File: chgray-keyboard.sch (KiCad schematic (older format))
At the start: 1 part

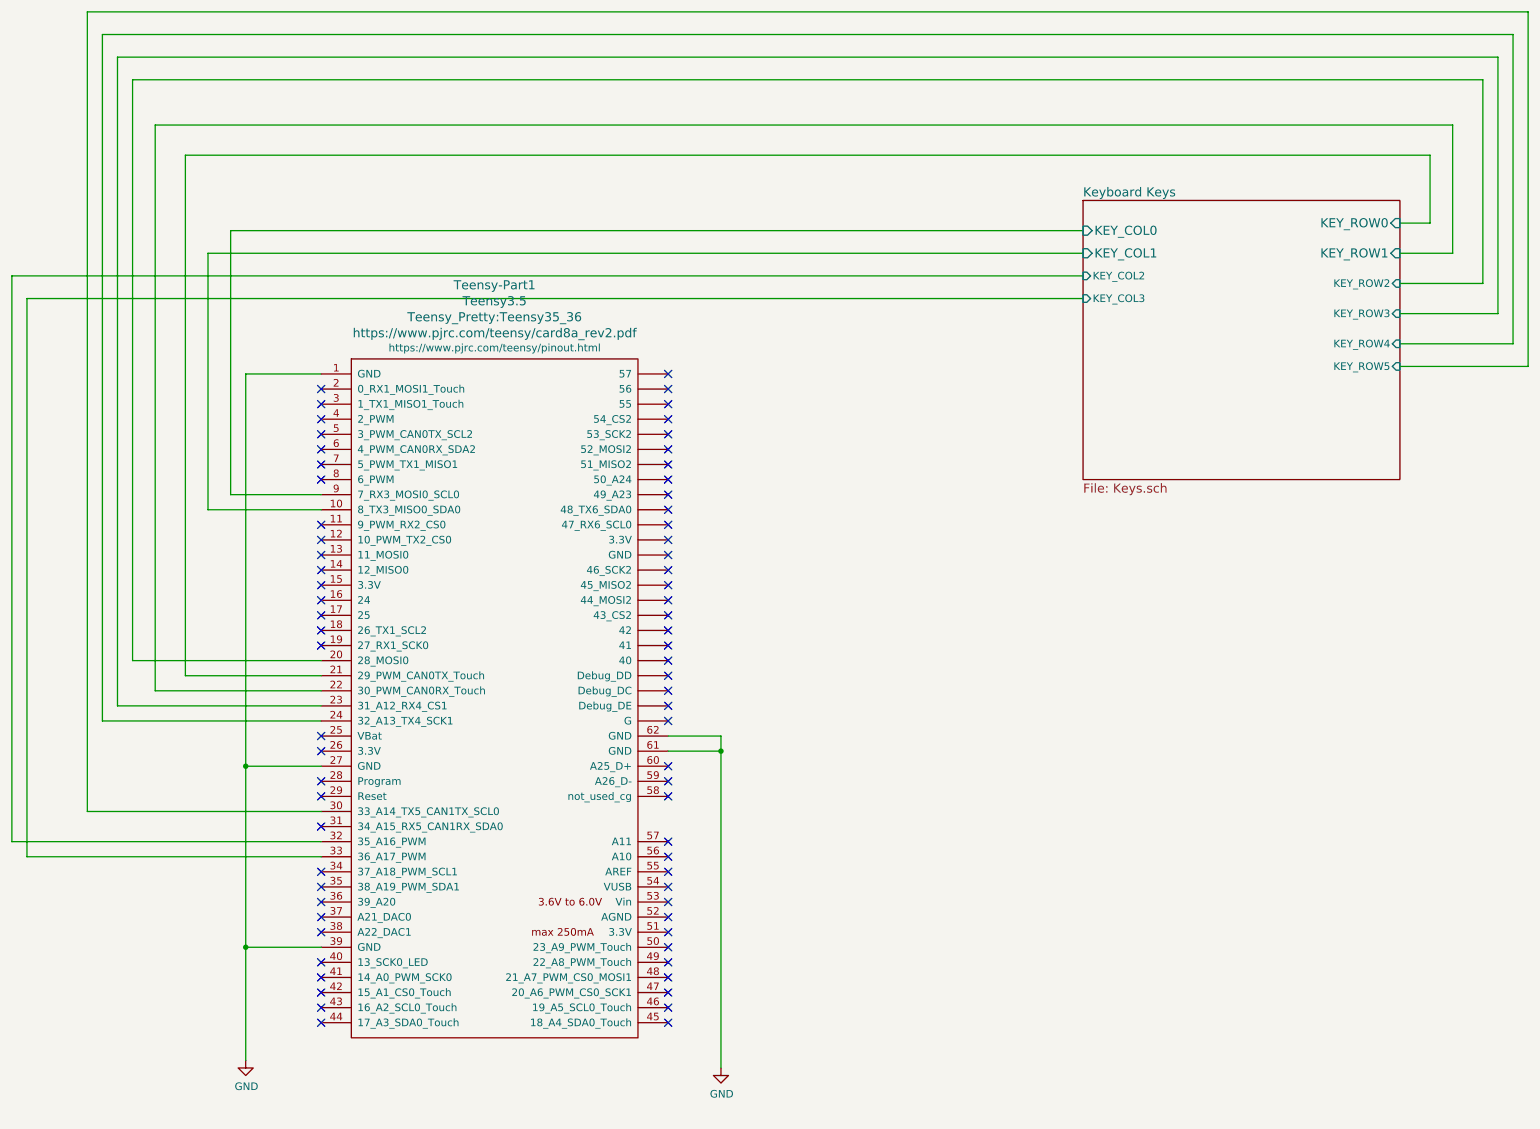
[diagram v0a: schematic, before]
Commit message: might work...
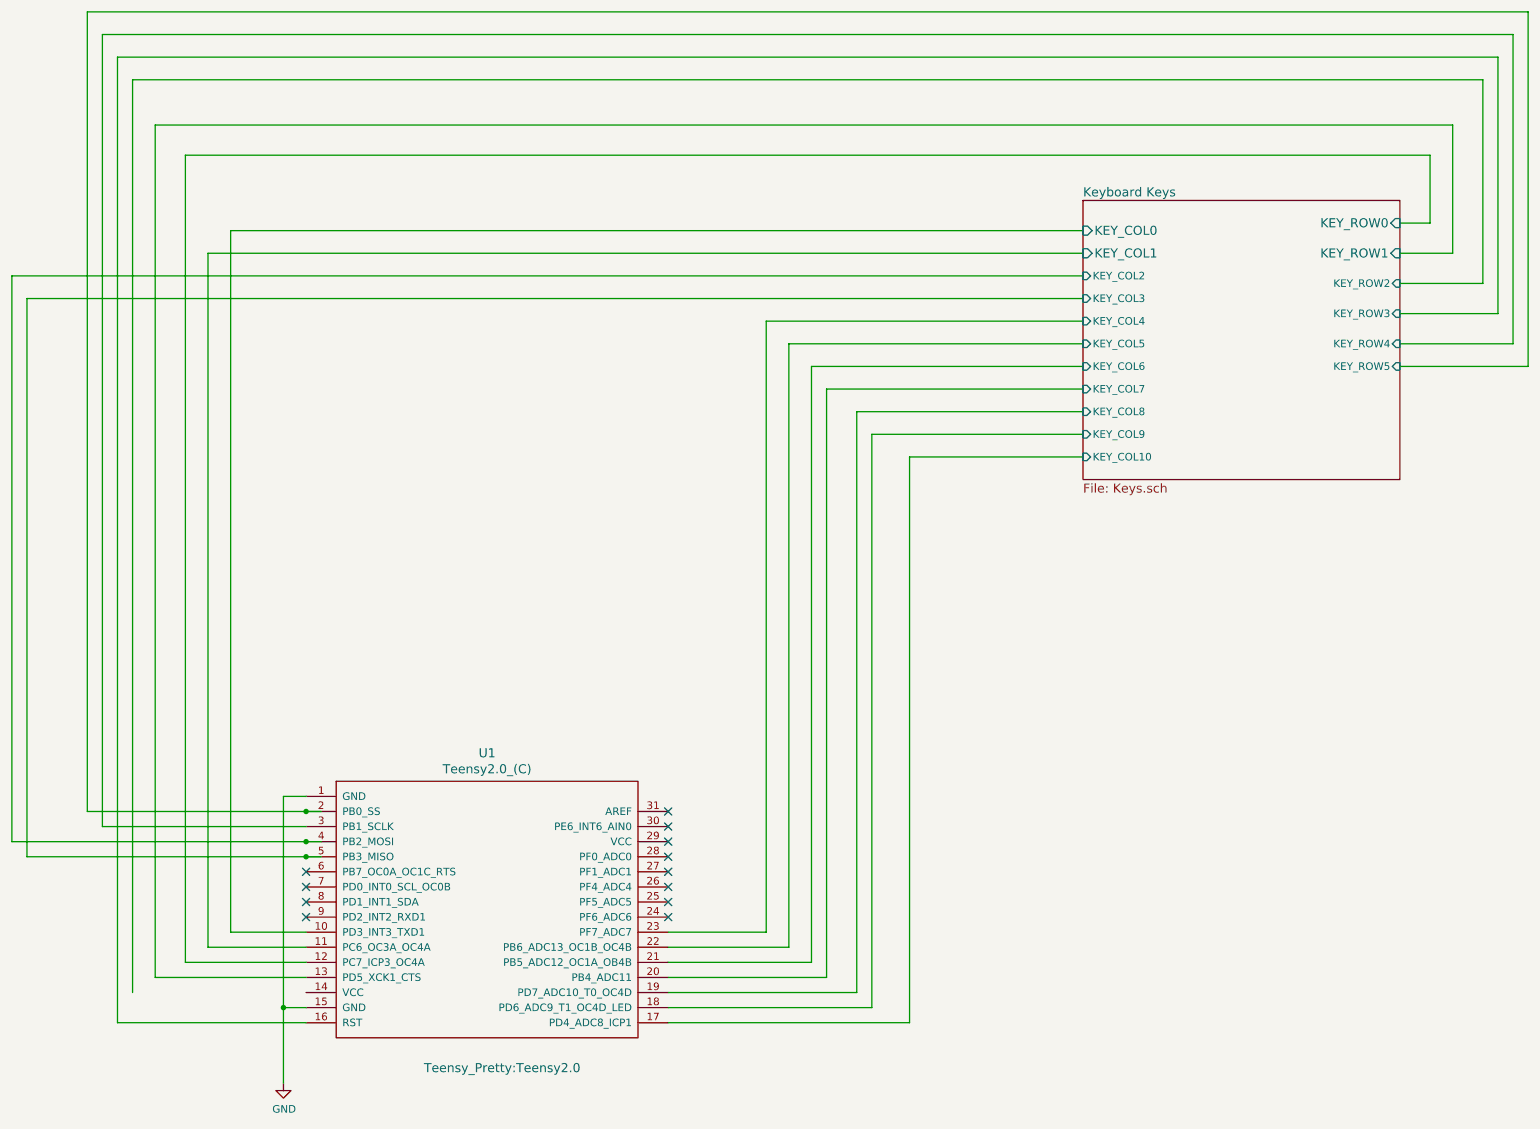
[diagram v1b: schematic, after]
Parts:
- removed Teensy-Part1: Teensy3.5, Teensy_Pretty:Teensy35_36, symbol chgray-keyboard-rescue:Teensy3.5-Teensy
- added U1: Teensy2.0_(C), Teensy_Pretty:Teensy2.0, symbol Teensy:Teensy2.0_(C)
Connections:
- wire segments 52 -> 69
- no-connect marks 71 -> 12
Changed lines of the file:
@@
 F10 "KEY_COL2" I L 7300 2300 50
 F11 "KEY_COL3" I L 7300 2450 50
+F12 "KEY_COL4" I L 7300 2600 50
+F13 "KEY_COL5" I L 7300 2750 50
+F14 "KEY_COL6" I L 7300 2900 50
+F15 "KEY_COL7" I L 7300 3050 50
+F16 "KEY_COL8" I L 7300 3200 50
+F17 "KEY_COL9" I L 7300 3350 50
+F18 "KEY_COL10" I L 7300 3500 50
 $EndSheet
 Wire Wire Line
@@
 	9600 1500 1350 1500
 Wire Wire Line
-	1350 1500 1350 4950
-Wire Wire Line
-	1150 5050 1150 1300
-Wire Wire Line
 	1150 1300 9750 1300
 Wire Wire Line
 	9750 1300 9750 2150
-Wire Wire Line
-	1350 4950 2250 4950
-Wire Wire Line
-	2250 5050 1150 5050
 Wire Wire Line
 	7300 2000 1650 2000
@@
 Wire Wire Line
 	9400 1950 9600 1950
-Wire Wire Line
-	1650 2000 1650 3750
-Wire Wire Line
-	1650 3750 2250 3750
-Wire Wire Line
-	2250 3850 1500 3850
-Wire Wire Line
-	1500 3850 1500 2150
 Wire Wire Line
 	1500 2150 7300 2150
@@
 	9950 1000 1000 1000
 Wire Wire Line
-	1000 1000 1000 4850
-Wire Wire Line
-	1000 4850 2250 4850
-NoConn ~ 4550 3850
-NoConn ~ 4550 3950
-NoConn ~ 4550 4050
-NoConn ~ 4550 4250
-NoConn ~ 4550 4350
-NoConn ~ 4550 4450
-NoConn ~ 4550 4550
-NoConn ~ 4550 4750
-NoConn ~ 4550 4850
-NoConn ~ 4550 4950
-NoConn ~ 4550 5050
-NoConn ~ 4550 5150
-NoConn ~ 4550 5250
-NoConn ~ 4550 5550
-NoConn ~ 4550 6050
-NoConn ~ 4550 6150
-NoConn ~ 4550 6250
-NoConn ~ 4550 6350
-NoConn ~ 4550 6450
-NoConn ~ 4550 6550
-NoConn ~ 4550 6650
-NoConn ~ 4550 6750
-NoConn ~ 4550 6850
-NoConn ~ 4550 6950
-NoConn ~ 4550 7050
-NoConn ~ 4550 7150
-NoConn ~ 4550 7250
-NoConn ~ 2250 7250
-NoConn ~ 2250 7150
-NoConn ~ 2250 7050
-NoConn ~ 2250 6950
-NoConn ~ 2250 6850
-NoConn ~ 2250 6650
-NoConn ~ 2250 6550
-NoConn ~ 2250 6450
-NoConn ~ 2250 6350
-NoConn ~ 2250 6250
-NoConn ~ 2250 5950
-NoConn ~ 2250 5750
-NoConn ~ 2250 5650
-NoConn ~ 2250 5450
-NoConn ~ 2250 4550
-NoConn ~ 2250 4650
-NoConn ~ 2250 4750
-NoConn ~ 2250 4450
-NoConn ~ 2250 4350
-NoConn ~ 2250 4250
-NoConn ~ 2250 4150
-NoConn ~ 2250 4050
-NoConn ~ 2250 3950
-NoConn ~ 2250 3650
-NoConn ~ 2250 3050
-NoConn ~ 2250 3150
-NoConn ~ 2250 3250
-NoConn ~ 2250 3350
-NoConn ~ 2250 3450
-NoConn ~ 2250 3550
-Wire Wire Line
 	9400 2550 10050 2550
 Wire Wire Line
@@
 Wire Wire Line
 	10050 850  900  850
-Wire Wire Line
-	900  850  900  5150
-Wire Wire Line
-	800  5250 800  700
 Wire Wire Line
 	800  700  10150 700
@@
 	10250 550  700  550
 Wire Wire Line
-	2250 5250 800  5250
+	10250 2900 9400 2900
 Wire Wire Line
-	900  5150 2250 5150
-Wire Wire Line
-	10250 2900 9400 2900
-NoConn ~ 2250 5350
-Wire Wire Line
-	2250 5850 700  5850
+	2250 5850 2150 5850
 Wire Wire Line
 	700  550  700  5850
-$Comp
-L chgray-keyboard-rescue:Teensy3.5-Teensy Teensy-Part1
-U 1 1 605697C1
-P 3400 5100
-F 0 "Teensy-Part1" H 3400 7839 60  0000 C CNN
-F 1 "Teensy3.5" H 3400 7733 60  0000 C CNN
-F 2 "Teensy_Pretty:Teensy35_36" H 3400 7627 60  0000 C CNN
-F 3 "https://www.pjrc.com/teensy/card8a_rev2.pdf" H 3400 7521 60  0000 C CNN
-F 4 "https://www.pjrc.com/teensy/pinout.html" H 3400 7423 50  0000 C CNN "Pinouts"
-	1    3400 5100
-	1    0    0    -1
-$EndComp
-NoConn ~ 4550 3150
-NoConn ~ 4550 3250
-NoConn ~ 4550 3350
-NoConn ~ 4550 3450
-NoConn ~ 4550 3550
-NoConn ~ 4550 5650
-NoConn ~ 4550 5750
-NoConn ~ 4550 4650
-$Comp
-L power:GND #PWR0101
-U 1 1 60644219
-P 1750 7500
-F 0 "#PWR0101" H 1750 7250 50  0001 C CNN
-F 1 "GND" H 1755 7327 50  0000 C CNN
-F 2 "" H 1750 7500 50  0001 C CNN
-F 3 "" H 1750 7500 50  0001 C CNN
-	1    1750 7500
-	1    0    0    -1
-$EndComp
 Wire Wire Line
-	2250 5550 1750 5550
-Wire Wire Line
-	1750 5550 1750 6750
-Wire Wire Line
-	2250 6750 1750 6750
-Connection ~ 1750 6750
-Wire Wire Line
-	1750 6750 1750 7500
-Wire Wire Line
-	2250 2950 1750 2950
-Wire Wire Line
-	1750 2950 1750 5550
-Connection ~ 1750 5550
-Wire Wire Line
-	4550 5350 4900 5350
-Wire Wire Line
-	4900 5350 4900 5450
-Wire Wire Line
-	4900 5450 4550 5450
-$Comp
-L power:GND #PWR0102
-U 1 1 6064C2E8
-P 4900 7550
-F 0 "#PWR0102" H 4900 7300 50  0001 C CNN
-F 1 "GND" H 4905 7377 50  0000 C CNN
-F 2 "" H 4900 7550 50  0001 C CNN
-F 3 "" H 4900 7550 50  0001 C CNN
-	1    4900 7550
-	1    0    0    -1
-$EndComp
-Wire Wire Line
-	4900 5450 4900 7550
-Connection ~ 4900 5450
-NoConn ~ 4550 2950
-NoConn ~ 4550 3050
-Wire Wire Line
-	2250 6050 200  6050
+	2250 6050 2150 6050
 Wire Wire Line
 	200  6050 200  2300
@@
 	300  2450 300  6150
 Wire Wire Line
-	300  6150 2250 6150
-NoConn ~ 4550 3650
-NoConn ~ 4550 3750
-NoConn ~ 4550 4150
+	300  6150 2150 6150
+Wire Wire Line
+	7300 2600 5200 2600
+Wire Wire Line
+	5200 2600 5200 6650
+Wire Wire Line
+	5200 6650 4550 6650
+Wire Wire Line
+	4550 6750 5350 6750
+Wire Wire Line
+	5350 6750 5350 2750
+Wire Wire Line
+	5350 2750 7300 2750
+Wire Wire Line
+	7300 2900 5500 2900
+Wire Wire Line
+	5500 2900 5500 6850
+Wire Wire Line
+	5500 6850 4550 6850
+Wire Wire Line
+	4550 6950 5600 6950
+Wire Wire Line
+	5600 6950 5600 3050
+Wire Wire Line
+	5600 3050 7300 3050
+Wire Wire Line
+	7300 3200 5800 3200
+Wire Wire Line
+	5800 3200 5800 7050
+Wire Wire Line
+	5800 7050 4550 7050
+Wire Wire Line
+	4550 7150 5900 7150
+Wire Wire Line
+	5900 7150 5900 3350
+Wire Wire Line
+	5900 3350 7300 3350
+Wire Wire Line
+	7300 3500 6150 3500
+Wire Wire Line
+	6150 3500 6150 7250
+Wire Wire Line
+	6150 7250 4550 7250
+$Comp
+L Teensy:Teensy2.0_(C) U1
+U 1 1 608F19B6
+P 3350 6500
+F 0 "U1" H 3350 7537 60  0000 C CNN
+F 1 "Teensy2.0_(C)" H 3350 7431 60  0000 C CNN
+F 2 "Teensy_Pretty:Teensy2.0" H 3450 5450 60  0000 C CNN
+F 3 "" H 3450 5450 60  0000 C CNN
+	1    3350 6500
+	1    0    0    -1
+$EndComp
+Connection ~ 2150 5850
+Wire Wire Line
+	2150 5850 700  5850
+Connection ~ 2150 6050
+Wire Wire Line
+	2150 6050 200  6050
+Connection ~ 2150 6150
+Wire Wire Line
+	2150 6150 2250 6150
+Wire Wire Line
+	900  7250 2150 7250
+Wire Wire Line
+	900  850  900  7250
+Wire Wire Line
+	1000 1000 1000 7050
+Wire Wire Line
+	1150 6950 2150 6950
+Wire Wire Line
+	1150 1300 1150 6950
+Wire Wire Line
+	1350 6850 2150 6850
+Wire Wire Line
+	1350 1500 1350 6850
+Wire Wire Line
+	1500 6750 2150 6750
+Wire Wire Line
+	1500 2150 1500 6750
+Wire Wire Line
+	1650 6650 2150 6650
+Wire Wire Line
+	1650 2000 1650 6650
+NoConn ~ 4550 5850
+NoConn ~ 4550 5950
+NoConn ~ 4550 6050
+NoConn ~ 4550 6150
+NoConn ~ 4550 6250
+NoConn ~ 4550 6350
+NoConn ~ 4550 6450
+NoConn ~ 4550 6550
+NoConn ~ 2150 6250
+NoConn ~ 2150 6350
+NoConn ~ 2150 6450
+NoConn ~ 2150 6550
+Wire Wire Line
+	2150 5950 800  5950
+Wire Wire Line
+	800  5950 800  700
+Wire Wire Line
+	2150 5750 2000 5750
+Wire Wire Line
+	2000 5750 2000 7150
+Wire Wire Line
+	2000 7150 2150 7150
+$Comp
+L power:GND #PWR0101
+U 1 1 6093A5EC
+P 2000 7650
+F 0 "#PWR0101" H 2000 7400 50  0001 C CNN
+F 1 "GND" H 2005 7477 50  0000 C CNN
+F 2 "" H 2000 7650 50  0001 C CNN
+F 3 "" H 2000 7650 50  0001 C CNN
+	1    2000 7650
+	1    0    0    -1
+$EndComp
+Wire Wire Line
+	2000 7150 2000 7650
+Connection ~ 2000 7150
 $EndSCHEMATC
